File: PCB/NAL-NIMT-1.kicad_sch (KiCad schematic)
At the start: 39 parts

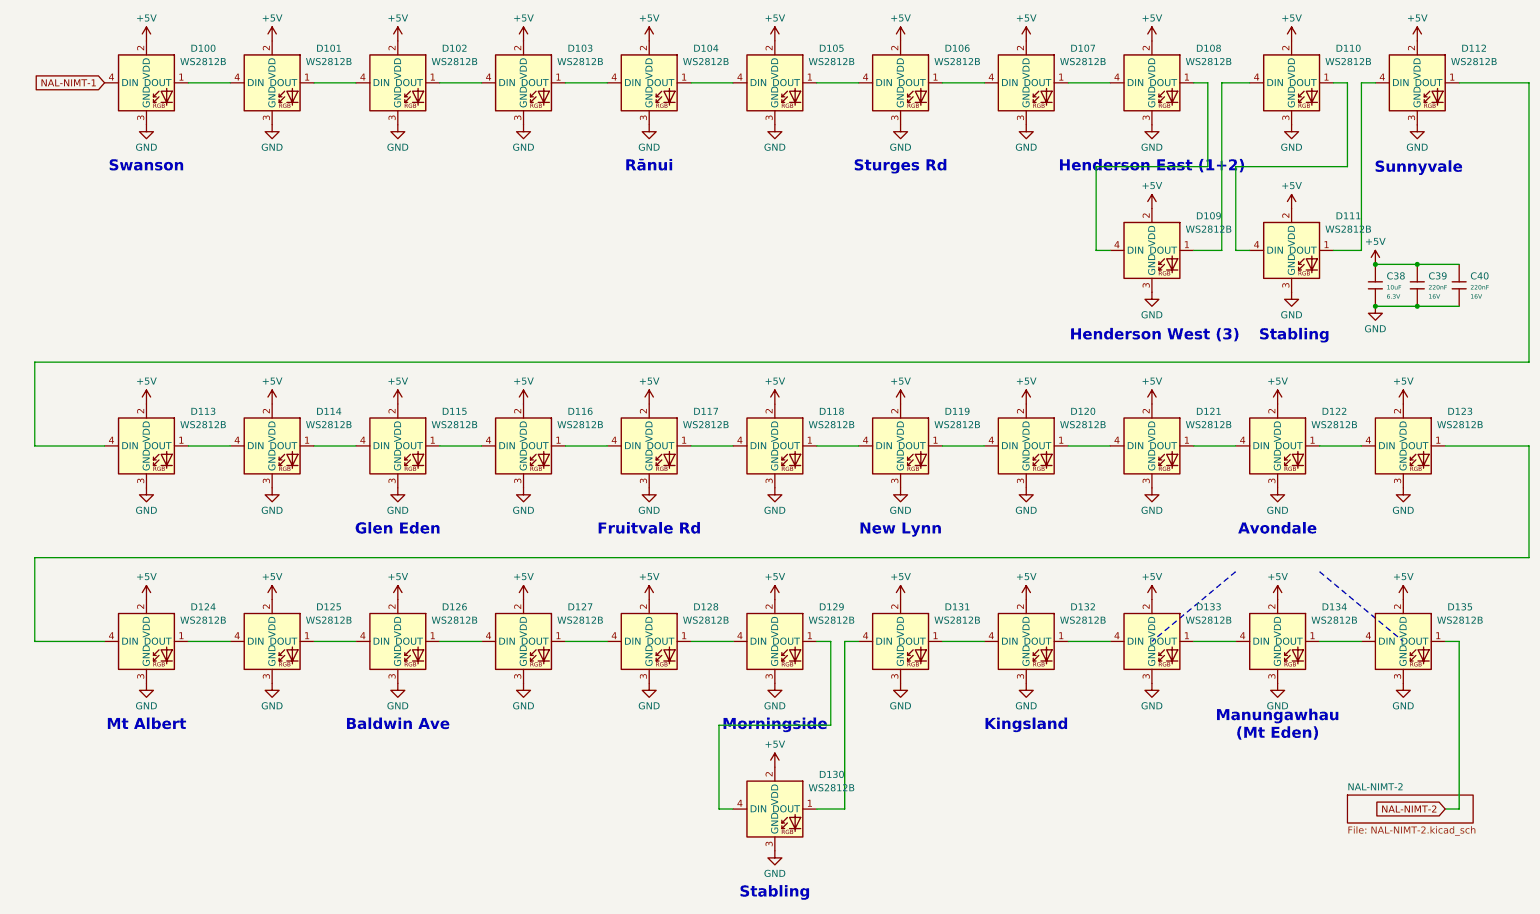
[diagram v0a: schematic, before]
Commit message: Final tweaks for V1.0.0
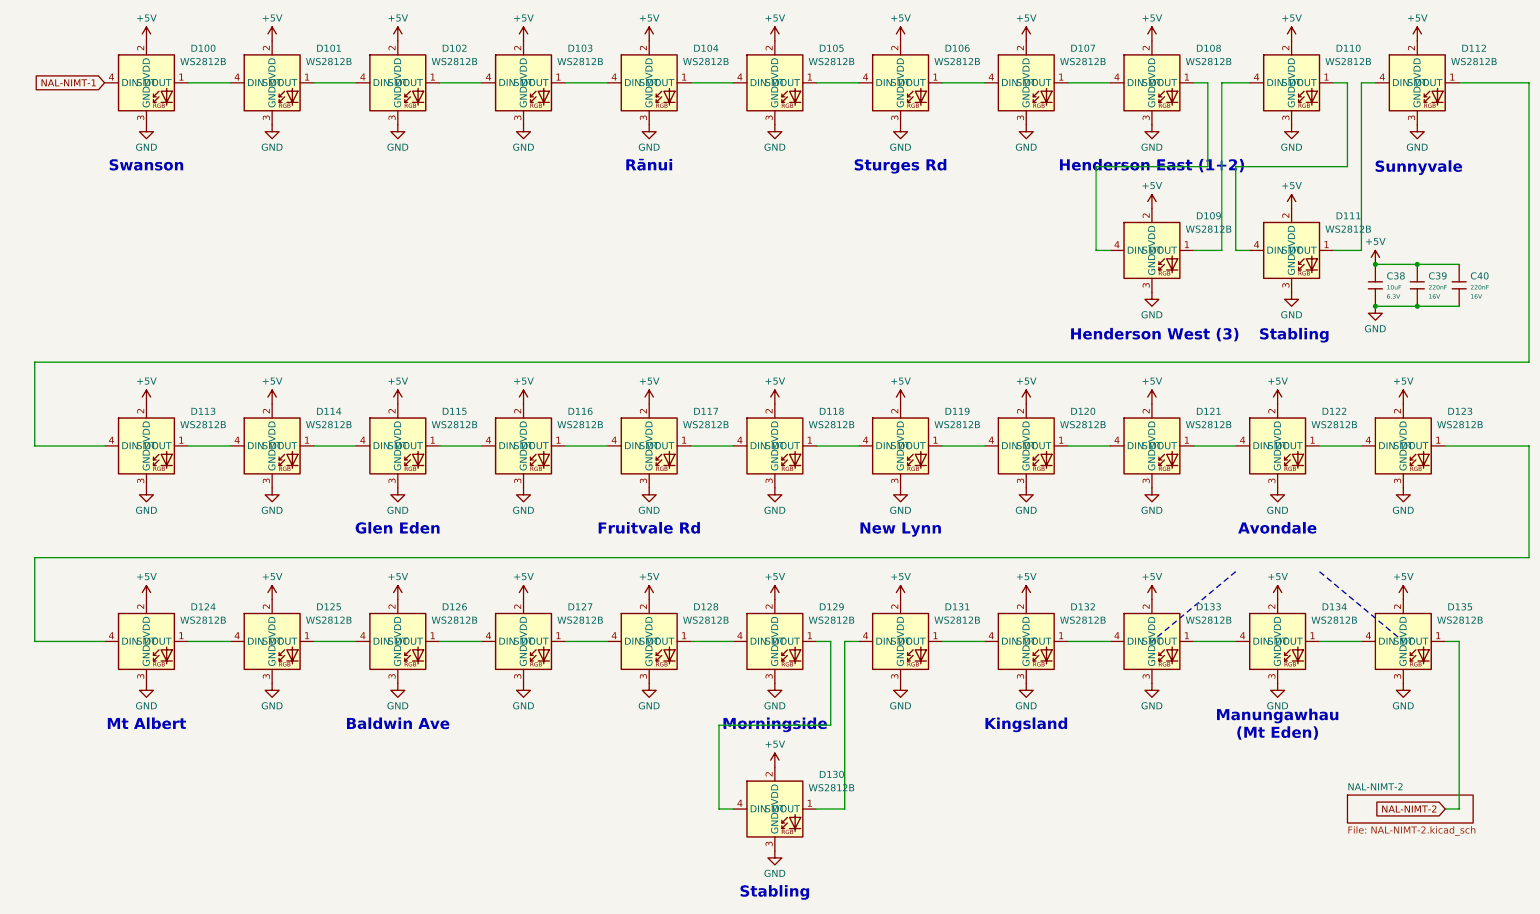
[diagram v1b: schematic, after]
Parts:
- D100, D101, D102, D103, D104, D105, D106, D107, D108, D109, D110, D111, D112, D113, D114, D115, D116, D117, D118, D119, D120, D121, D122, D123, D124, D125, D126, D127, D128, D129, D130, D131, D132, D133, D134, D135: Manufacturer (none) -> XINGLIGHT; Part (none) -> XL-1615RGBC-WS2812B; Process (none) -> SMT

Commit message: V1.1.0 PCB
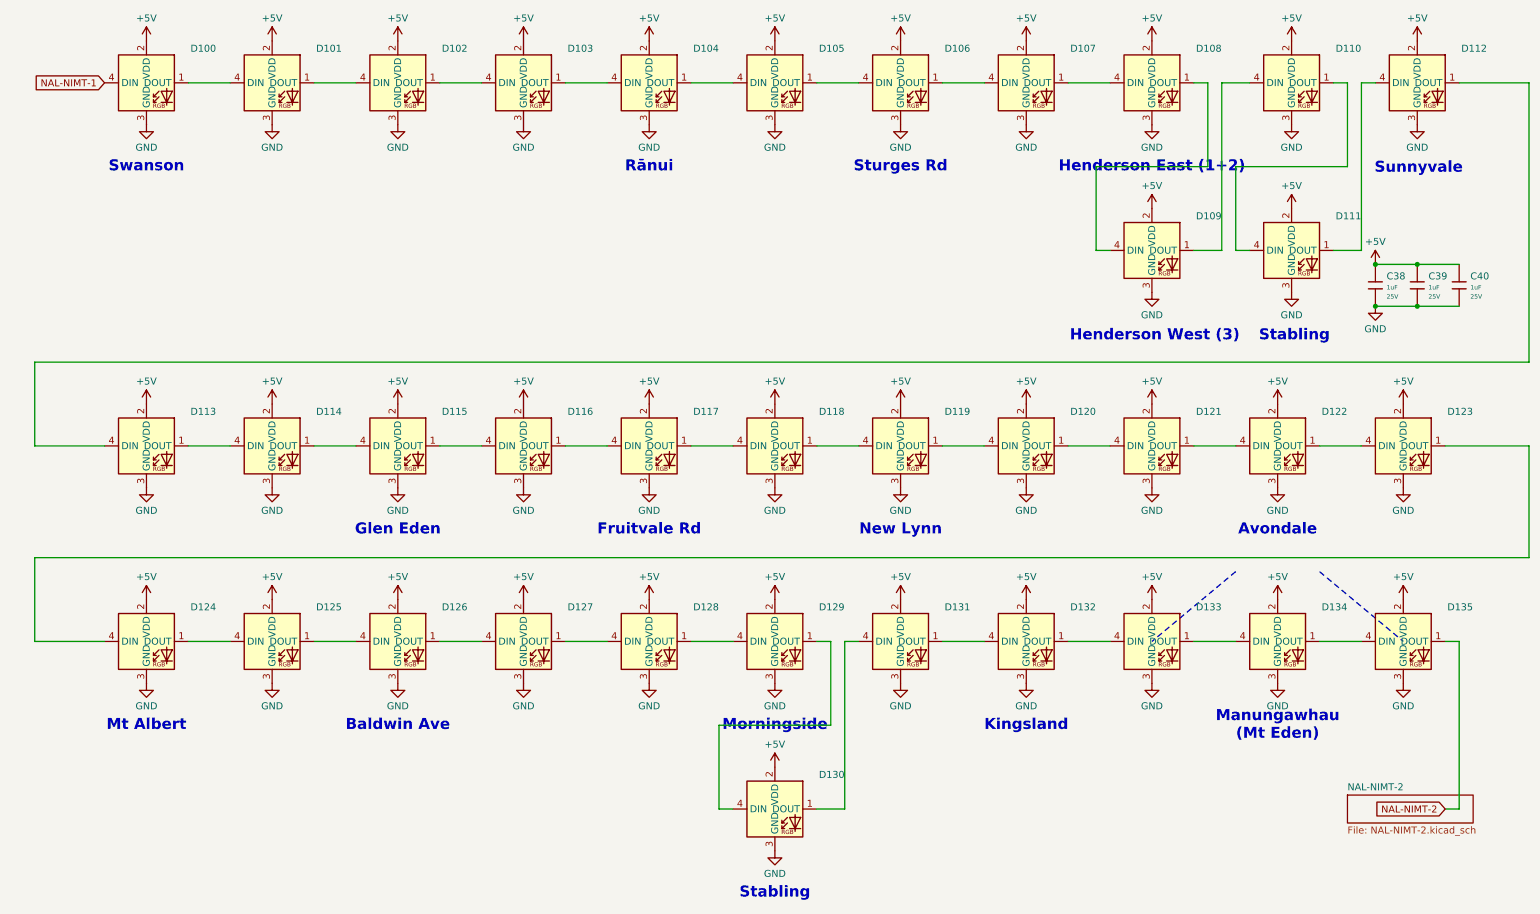
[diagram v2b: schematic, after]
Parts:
- C38: value 10uF -> 1uF; symbol PCM_JLCPCB-Capacitors:0402,10uF -> PCM_JLCPCB-Capacitors:0402,1uF; Capacitance 10uF -> 1uF; LCSC C15525 -> C52923; Part CL05A106MQ5NUNC -> CL05A105KA5NQNC; Price 0.007USD -> 0.006USD; Stock 1595146 -> 9606588; Tolerance ±20% -> ±10%; Voltage Rated 6.3V -> 25V
- C39, C40: value 220nF -> 1uF; symbol PCM_JLCPCB-Capacitors:0402,220nF -> PCM_JLCPCB-Capacitors:0402,1uF; Capacitance 220nF -> 1uF; LCSC C16772 -> C52923; Part CL05B224KO5NNNC -> CL05A105KA5NQNC; Price 0.008USD -> 0.006USD; Stock 351761 -> 9606588; Temperature Coefficient X7R -> X5R; Voltage Rated 16V -> 25V
- D100, D101, D102, D103, D104, D105, D106, D107, D108, D109, D110, D111, D112, D113, D114, D115, D116, D117, D118, D119, D120, D121, D122, D123, D124, D125, D126, D127, D128, D129, D130, D131, D132, D133, D134, D135: value WS2812B -> XL-1615RGBC-WS2812B-S; LCSC C5349954 -> C41413180; Manufacturer XINGLIGHT -> (none); Part XL-1615RGBC-WS2812B -> (none); Process SMT -> (none)

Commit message: Update to meet OSHWA Certification
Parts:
- D100, D101, D102, D103, D104, D105, D106, D107, D108, D109, D110, D111, D112, D113, D114, D115, D116, D117, D118, D119, D120, D121, D122, D123, D124, D125, D126, D127, D128, D129, D130, D131, D132, D133, D134, D135: Manufacturer (none) -> XINGLIGHT; Part (none) -> XL-1615RGBC-WS2812B-S
